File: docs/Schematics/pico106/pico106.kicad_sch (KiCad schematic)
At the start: 18 parts, among them J1 MIDI in, J2 Debug, J3 Stereo line out, J4 Debug, J6 Stereo line out, SW1 RST, U1 Pico 2 (RP2350), U3 H11L1

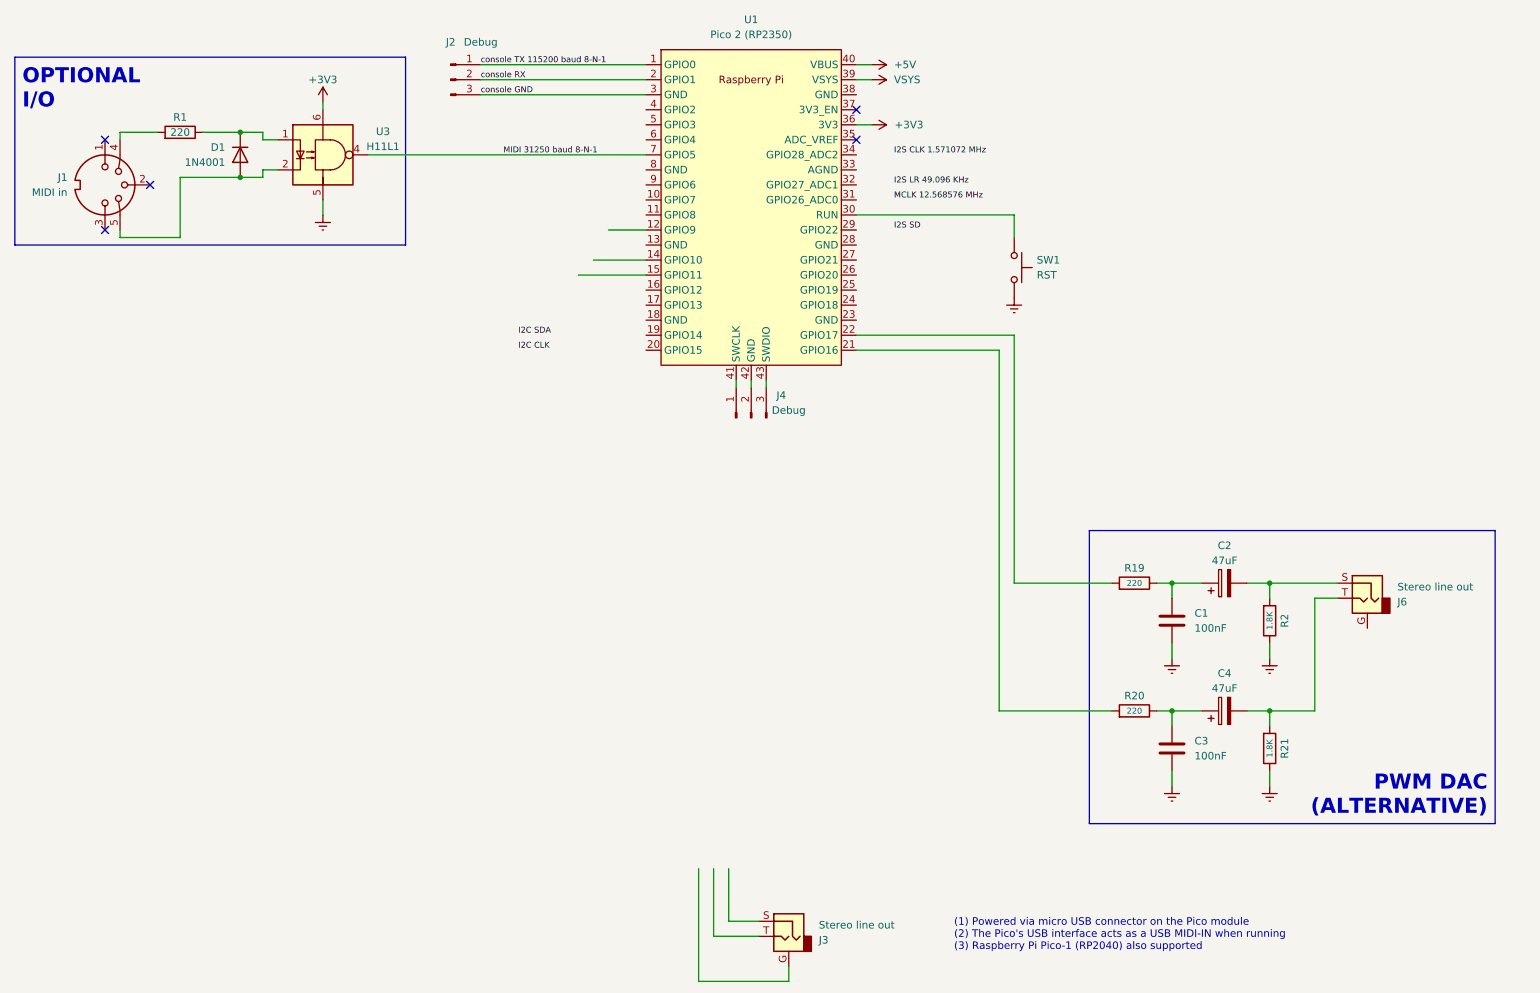
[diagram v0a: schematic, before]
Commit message: Update schematic
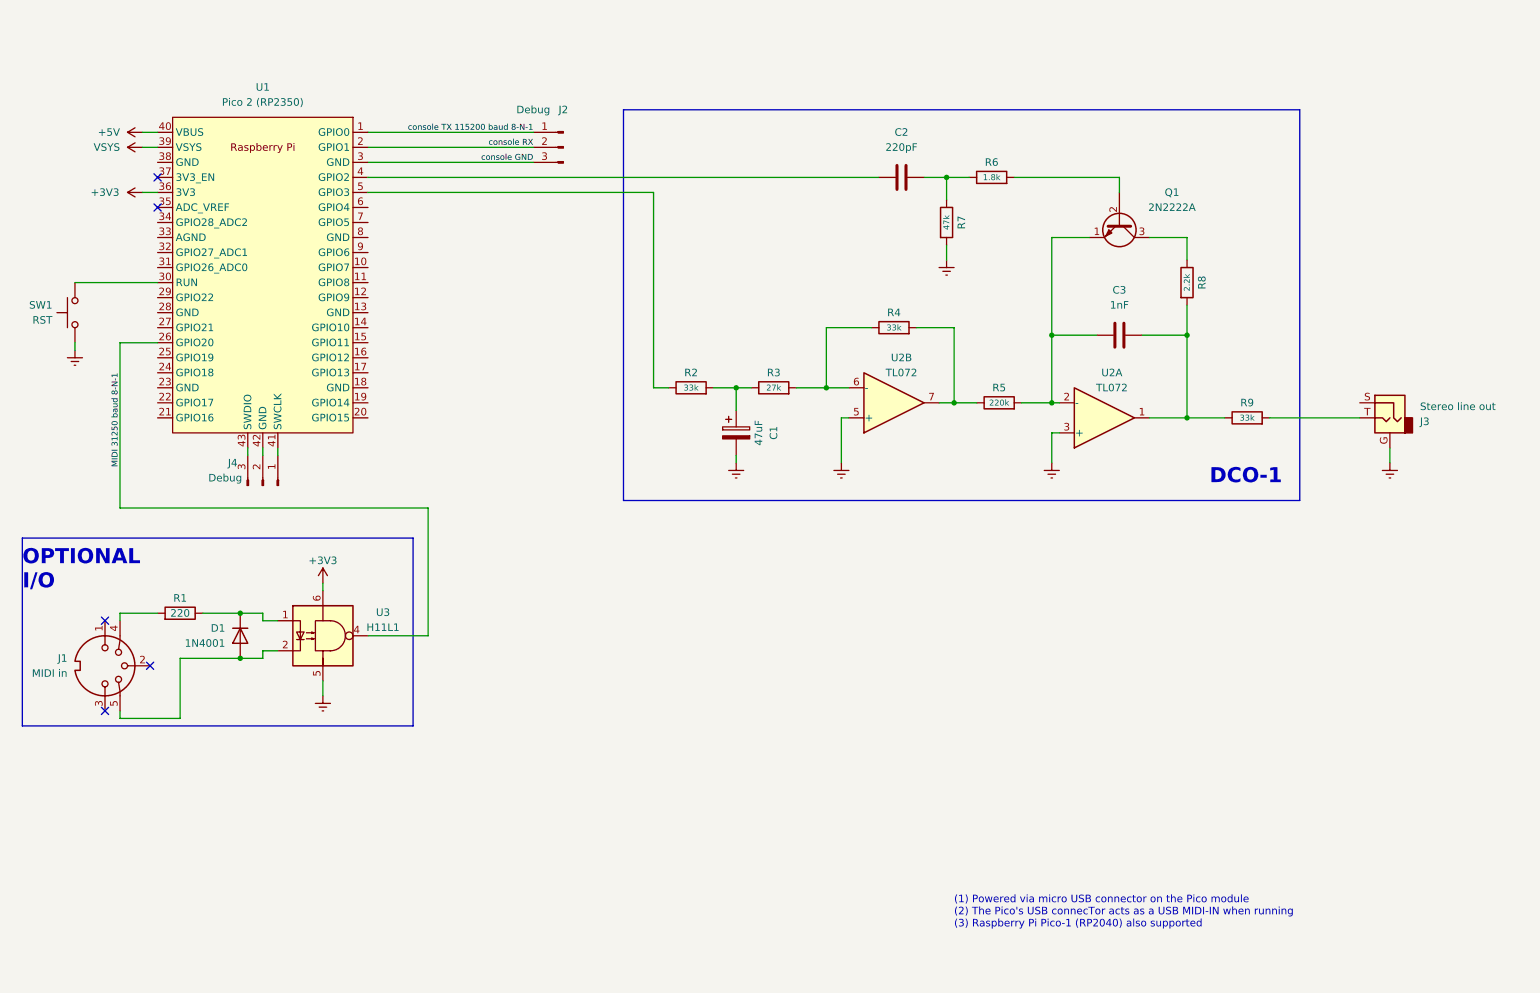
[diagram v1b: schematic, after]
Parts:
- removed C1: 100nF, symbol Device:C
- removed C2, C4: 47uF, symbol Device:C_Polarized
- removed J6: Stereo line out, Connector_Audio:Jack_3.5mm_CUI_SJ1-3523N_Horizontal, symbol Connector_Audio:AudioJack2_Ground
- removed R19, R20: 220, Resistor_THT:R_Axial_DIN0204_L3.6mm_D1.6mm_P5.08mm_Horizontal, symbol Device:R
- removed R21: 1.8K, Resistor_THT:R_Axial_DIN0204_L3.6mm_D1.6mm_P5.08mm_Horizontal, symbol Device:R
- added C1: 47uF, symbol Device:C_Polarized
- added C2: 220pF, symbol Device:C
- added Q1: 2N2222A, Package_TO_SOT_THT:TO-39-3, symbol Transistor_BJT:2N2219
- added R3: 27k, Resistor_THT:R_Axial_DIN0204_L3.6mm_D1.6mm_P5.08mm_Horizontal, symbol Device:R
- added R4, R9: 33k, Resistor_THT:R_Axial_DIN0204_L3.6mm_D1.6mm_P5.08mm_Horizontal, symbol Device:R
- added R5: 220k, Resistor_THT:R_Axial_DIN0204_L3.6mm_D1.6mm_P5.08mm_Horizontal, symbol Device:R
- added R6: 1.8k, Resistor_THT:R_Axial_DIN0204_L3.6mm_D1.6mm_P5.08mm_Horizontal, symbol Device:R
- added R7: 47k, esistor_THT:R_Axial_DIN0204_L3.6mm_D1.6mm_P5.08mm_Horizontal, symbol Device:R
- added R8: 2.2k, Resistor_THT:R_Axial_DIN0204_L3.6mm_D1.6mm_P5.08mm_Horizontal, symbol Device:R
- added U2: TL072, symbol Amplifier_Operational:TL072
- C3: value 100nF -> 1nF
- R2: value 1.8K -> 33k
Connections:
- net Earth: now also J3.G, C1.2, R7.2, U2.3 (+), U2.5 (+); no longer C3.2, R2.1
- net MIDI 31250 baud 8-N-1: now also U1.26 (GPIO20); no longer U1.7 (GPIO5)
- net at U1.4 (GPIO2): now also C2.1
- net at U1.5 (GPIO3): now also R2.1
- net at C3.1: now also Q1.1 (E), R5.2, U2.2 (-)
- net at J3.T: now also R9.2
- net at R2.2: now also C1.1, R3.1
- new net: C2.2, R6.1, R7.1
- new net: C3.2, R8.2, R9.1, U2.1
- new net: R4.2, R5.1, U2.7
- new net: Q1.3 (C), R8.1
- new net: Q1.2 (B), R6.2
- new net: R3.2, R4.1, U2.6 (-)
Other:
- note added: "(1) Powered via micro USB connector on the Pico module (2) The Pico's USB connecTor acts as a USB MIDI-IN when running (3) Raspberry Pi Pico-1 (RP2040) also supported"
- note added: "DCO-1"
- note removed: "(1) Powered via micro USB connector on the Pico module (2) The Pico's USB interface acts as a USB MIDI-IN when running (3) Raspberry Pi Pico-1 (RP2040) also supported"
- note removed: "PWM DAC (ALTERNATIVE)"
- moved on the sheet: D1, J1, J2, J3, J4, R1, SW1, U1, U3
